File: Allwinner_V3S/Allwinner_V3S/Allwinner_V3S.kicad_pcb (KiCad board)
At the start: 2 copper layers, 33 parts, among them U1 Allwinner_V3S, U2 SY8088AAC, U3 SY8088AAC, U4 SY8088AAC, U5 CH340N, Y1 24M

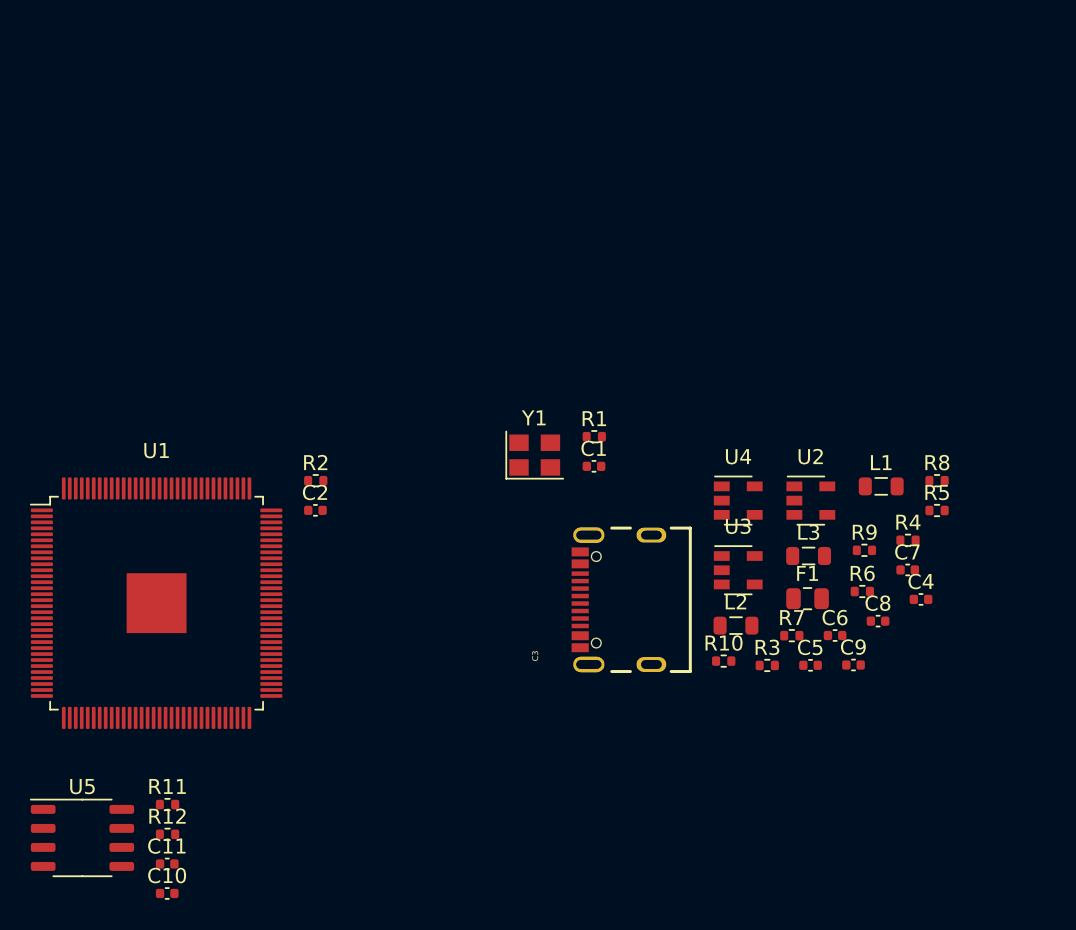
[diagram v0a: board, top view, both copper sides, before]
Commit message: update
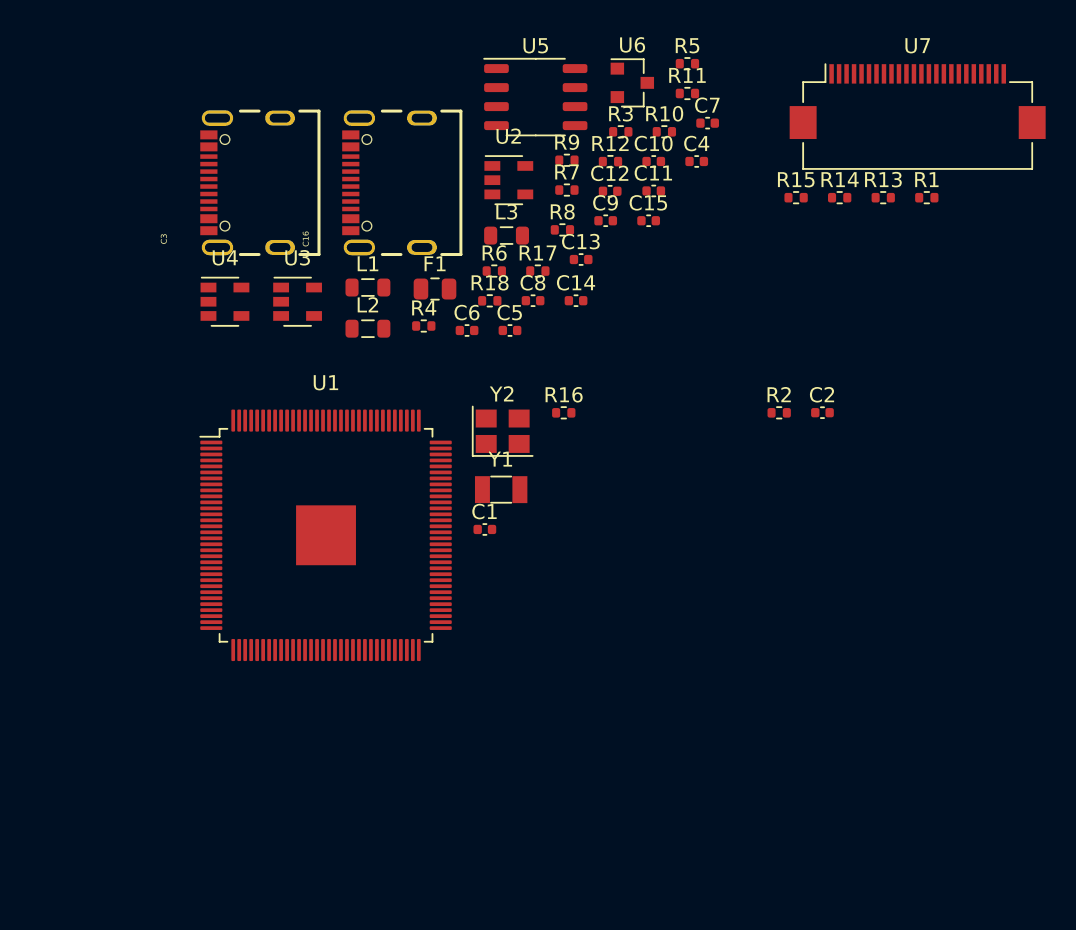
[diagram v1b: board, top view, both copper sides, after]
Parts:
- added C12: 104, Capacitor_SMD:C_0402_1005Metric, F.Cu at (144.8, 73.4)
- added C13: 106, Capacitor_SMD:C_0402_1005Metric, F.Cu at (142.9, 78.0)
- added C14: 104, Capacitor_SMD:C_0402_1005Metric, F.Cu at (142.6, 80.8)
- added C15: 106, Capacitor_SMD:C_0402_1005Metric, F.Cu at (147.4, 75.4)
- added C16: USB-TypeC-16Pin, mypack:USB-TYPT-C-16PIN, F.Cu at (131.0, 72.9)
- added R13: 10K, Resistor_SMD:R_0402_1005Metric, F.Cu at (163.1, 73.9)
- added R14: 10K, Resistor_SMD:R_0402_1005Metric, F.Cu at (160.2, 73.9)
- added R15: 10K, Resistor_SMD:R_0402_1005Metric, F.Cu at (157.3, 73.9)
- added R16: 240, Resistor_SMD:R_0402_1005Metric, F.Cu at (141.7, 88.2)
- added R17: 22, Resistor_SMD:R_0402_1005Metric, F.Cu at (140.0, 78.8)
- added R18: 22, Resistor_SMD:R_0402_1005Metric, F.Cu at (136.8, 80.8)
- added U6: XC6206PxxxMR, Package_TO_SOT_SMD:SOT-23, F.Cu at (146.3, 66.2)
- added U7: FPC_24, mypack:Hirose_FH12-24S-0.5SH_1x24-1MP_P0.50mm_Horizontal, F.Cu at (165.4, 67.5)
- added Y2: 24M, Crystal:Crystal_SMD_3225-4Pin_3.2x2.5mm, F.Cu at (137.7, 89.5)
- R1: value 240 -> 10K
- Y1: value 24M -> 32.768K; footprint Oscillator:Oscillator_SMD_Abracon_ASE-4Pin_3.2x2.5mm -> Crystal:Crystal_SMD_3215-2Pin_3.2x1.5mm
- moved R11 58.8 mm to (150.0, 66.9)
- moved C10 58.7 mm to (147.8, 71.5)
- moved U5 58.0 mm to (139.9, 67.2)
- moved C11 55.5 mm to (147.8, 73.4)
- moved R12 53.8 mm to (144.9, 71.5)
- moved C3 37.3 mm to (121.5, 72.9)
- moved R3 37.0 mm to (145.6, 69.5)
- moved L1 36.8 mm to (128.7, 79.9)
- moved U4 36.8 mm to (119.1, 80.8)
- moved R10 35.6 mm to (148.5, 69.5)
- moved R4 35.4 mm to (132.4, 82.4)
- moved C2 34.5 mm to (159.0, 88.2)
- moved U3 34.5 mm to (124.0, 80.8)
- moved R5 34.2 mm to (150.0, 64.9)
- moved C9 34.0 mm to (144.5, 75.4)
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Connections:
- net /DRAM_VREF renamed /v3s_core/DRAM_VREF
- net /RESET renamed /v3s_core/RESET
- C3 pad A6: /USB_DP -> /power/USB0_DP
- C3 pad A7: /USB_DN -> /power/USB0_DN
- C3 pad B6: /USB_DP -> /power/USB0_DP
- C3 pad B7: /USB_DN -> /power/USB0_DN
- R1 pad 2: GND -> +2V8
- R11 pad 1: /usb_uart/USB_RXD -> /v3s_core/PB8_TWI1_SCK_UART0_TX_PB_EINT8
- R12 pad 1: /usb_uart/USB_TXD -> /v3s_core/PB9_TWI1_SDA_UART0_RX_PB_EINT9
- R3 pad 1: /USB_DP -> Net-(R3-Pad1)
- R3 pad 2: /USB_DP -> /power/USB0_DP
- R4 pad 1: /USB_DN -> Net-(R4-Pad1)
- R4 pad 2: /USB_DN -> /power/USB0_DN
- U1 pad 109: Net-(U1-Pad109) -> +3V3
- U1 pad 110: Net-(U1-Pad110) -> /power/USB1_DN
- U1 pad 111: Net-(U1-Pad111) -> /power/USB1_DP
- U1 pad 115: Net-(U1-Pad115) -> +3V0
- U1 pad 116: Net-(U1-Pad116) -> GND
- U1 pad 122: Net-(U1-Pad122) -> +3V3
- U1 pad 16: Net-(U1-Pad16) -> /camera_fpc24/PE15_CSI_D11_LCD_D15
- U1 pad 17: Net-(U1-Pad17) -> /camera_fpc24/PE14_CSI_D10_LCD_D14
- U1 pad 18: Net-(U1-Pad18) -> /camera_fpc24/PE13_CSI_D9_LCD_D13
- U1 pad 22: Net-(U1-Pad22) -> /camera_fpc24/PE12_CSI_D8_LCD_D12
- U1 pad 23: Net-(U1-Pad23) -> /camera_fpc24/PE11_CSI_D7_LCD_D11
- U1 pad 24: Net-(U1-Pad24) -> /camera_fpc24/PE10_CSI_D7_LCD_D10
- U1 pad 27: Net-(U1-Pad27) -> /camera_fpc24/PE9_CSI_D5_LCD7
- U1 pad 28: Net-(U1-Pad28) -> /camera_fpc24/PE8_CSI_D4_LCD_D6
- U1 pad 34: Net-(U1-Pad34) -> /camera_fpc24/PE3_CSI_VSYNCLCD_VSYNC
- U1 pad 35: Net-(U1-Pad35) -> /camera_fpc24/PE2_CSI_HSYSNC_LCD_HSYNC
- U1 pad 36: Net-(U1-Pad36) -> /camera_fpc24/PE1_CSI_MCLK_LCD_DE
- U1 pad 37: Net-(U1-Pad37) -> /camera_fpc24/PE0_CSI_PCLK_LCD_CLK
- U1 pad 48: Net-(U1-Pad48) -> /v3s_core/PB8_TWI1_SCK_UART0_TX_PB_EINT8
- U1 pad 49: Net-(U1-Pad49) -> /v3s_core/PB9_TWI1_SDA_UART0_RX_PB_EINT9
- U1 pad 73: Net-(R1-Pad1) -> Net-(R16-Pad1)
- U1 pad 8: Net-(U1-Pad8) -> /camera_fpc24/PE22_CSI_SDA_TWI1_SDA_UART1_RX
- U1 pad 85: Net-(U1-Pad85) -> +3V3
- U1 pad 88: Net-(U1-Pad88) -> +1V2
- U1 pad 9: Net-(U1-Pad9) -> /camera_fpc24/PE21_CSI_SCK_TWI1_SCK_UART1_TX
- U5 pad 1: /USB_DP -> Net-(R3-Pad1)
- U5 pad 2: /USB_DN -> Net-(R4-Pad1)
- Y1 pad 1: Net-(U1-Pad74) -> Net-(U1-Pad96)
- Y1 pad 2: GND -> Net-(Y1-Pad2)
